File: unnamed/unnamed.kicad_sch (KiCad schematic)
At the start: 128 parts, among them J1 Serial, J2 Serial, J3 Conn_01x01_Female, J4 Conn_01x01_Female, J5 S3B-PH-SM4-TB(LF)(SN), J6 S3B-PH-SM4-TB(LF)(SN), J7 Conn_01x12_Female, J8 Conn_01x12_Female, SW1 SW_Push, SW10 SW_Push, SW11 SW_Push, SW12 SW_Push, SW13 SW_Push, SW14 SW_Push, SW15 SW_Push, SW16 SW_Push, SW17 SW_Push, SW18 SW_Push, SW19 SW_Push, SW2 SW_Push, SW20 SW_Push, SW21 SW_Push, SW22 SW_Push, SW23 SW_Push, SW24 SW_Push, SW25 SW_SPST, SW26 SW_SPST, SW27 SW_Push, SW28 SW_Push, SW29 SW_Push, SW3 SW_Push, SW30 SW_Push, SW31 SW_Push, SW32 SW_Push, SW33 SW_Push, SW34 SW_Push, SW35 SW_Push, SW36 SW_Push, SW4 SW_Push, SW5 SW_Push, SW6 SW_Push, SW7 SW_Push, SW8 SW_Push, SW9 SW_Push, U1 eliteC, U2 eliteC

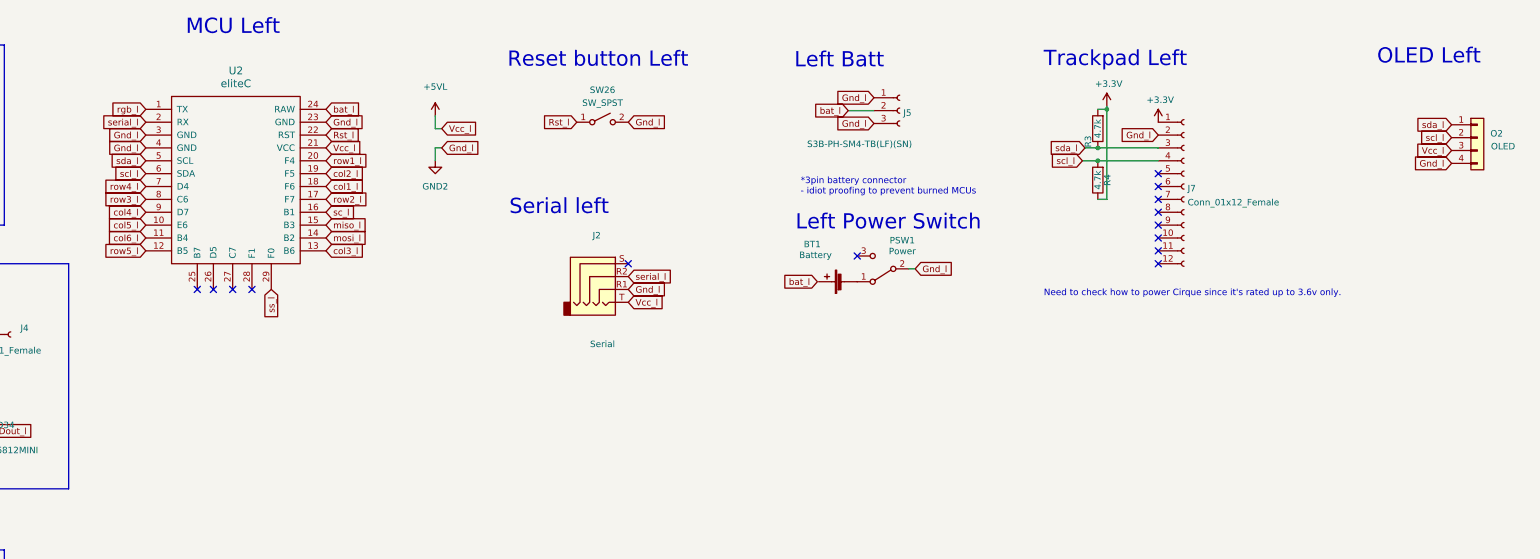
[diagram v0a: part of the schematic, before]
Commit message: routing
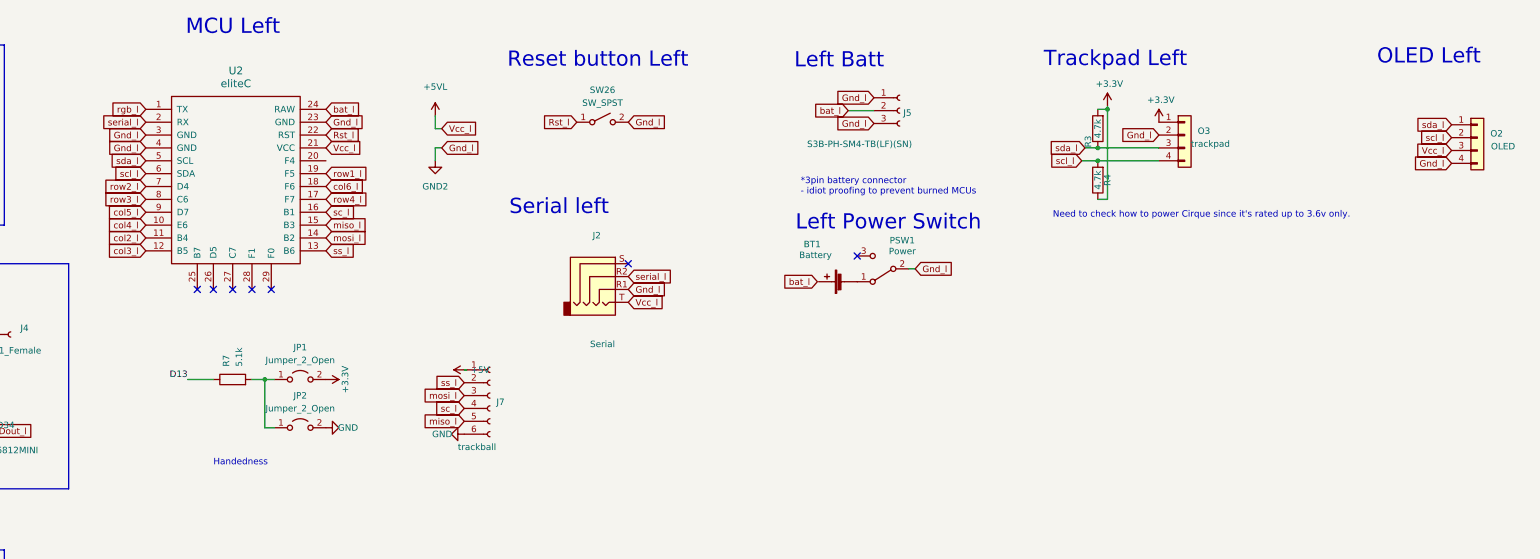
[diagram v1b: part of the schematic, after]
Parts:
- removed J7: Conn_01x12_Female, prettylib:FPC-SMD_FH12-12S-0.5SH-55, symbol Connector:Conn_01x12_Female
- added J7: trackball, Library:6_PinHeader, symbol Connector:Conn_01x06_Female
- added JP1, JP2: Jumper_2_Open, Library:SolderJumper-2_P1.3mm_Open_RoundedPad1.0x1.5mm, symbol Jumper:Jumper_2_Open
- added O3: trackpad, Connector_PinHeader_2.54mm:PinHeader_1x04_P2.54mm_Vertical, symbol Connector_Generic:Conn_01x04
- added R7: 5.1k, Resistor_SMD:R_0402_1005Metric, symbol Device:R
- U2: footprint (none) -> Library:Elite-C
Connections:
- net col1_l is gone; now on net col6_l: U2.18 (F6)
- net row5_l is gone; now on net col3_l: U2.12 (B5)
- net +3V3: now also JP1.2 (B), O3.1 (Pin_1)
- net +5V: now also J7.1 (Pin_1)
- net GND: now also J7.6 (Pin_6), JP2.2 (B)
- net GND2: now also O3.2 (Pin_2)
- net col2_l: now also U2.11 (B4); no longer U2.19 (F5)
- net col3_l: no longer U2.13 (B6)
- net col4_l: now also U2.10 (E6); no longer U2.9 (D7)
- net col5_l: now also U2.9 (D7); no longer U2.10 (E6)
- net col6_l: no longer U2.11 (B4)
- net miso_l: now also J7.5 (Pin_5)
- net mosi_l: now also J7.3 (Pin_3)
- net row1_l: now also U2.19 (F5); no longer U2.20 (F4)
- net row2_l: now also U2.7 (D4); no longer U2.17 (F7)
- net row4_l: now also U2.17 (F7); no longer U2.7 (D4)
- net sc_l: now also J7.4 (Pin_4)
- net scl_l: now also O3.4 (Pin_4)
- net sda_l: now also O3.3 (Pin_3)
- net ss_l: now also U2.13 (B6), J7.2 (Pin_2); no longer U2.29 (F0)
- new net: JP1.1 (A), JP2.1 (A), R7.2
- new net D13: R7.1
- no-connect marks 28 -> 21
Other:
- note added: "Handedness"
